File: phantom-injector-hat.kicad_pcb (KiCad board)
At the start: 2 copper layers, 65 x 44.8 mm, 42 parts, among them J1 Conn_02x20_Odd_Even, J2 Conn_02x03_Top_Bottom, J3 Conn_01x03, J4 Conn_01x03, SW1 SW_SPST, U1 LT8362EMSE-PBF

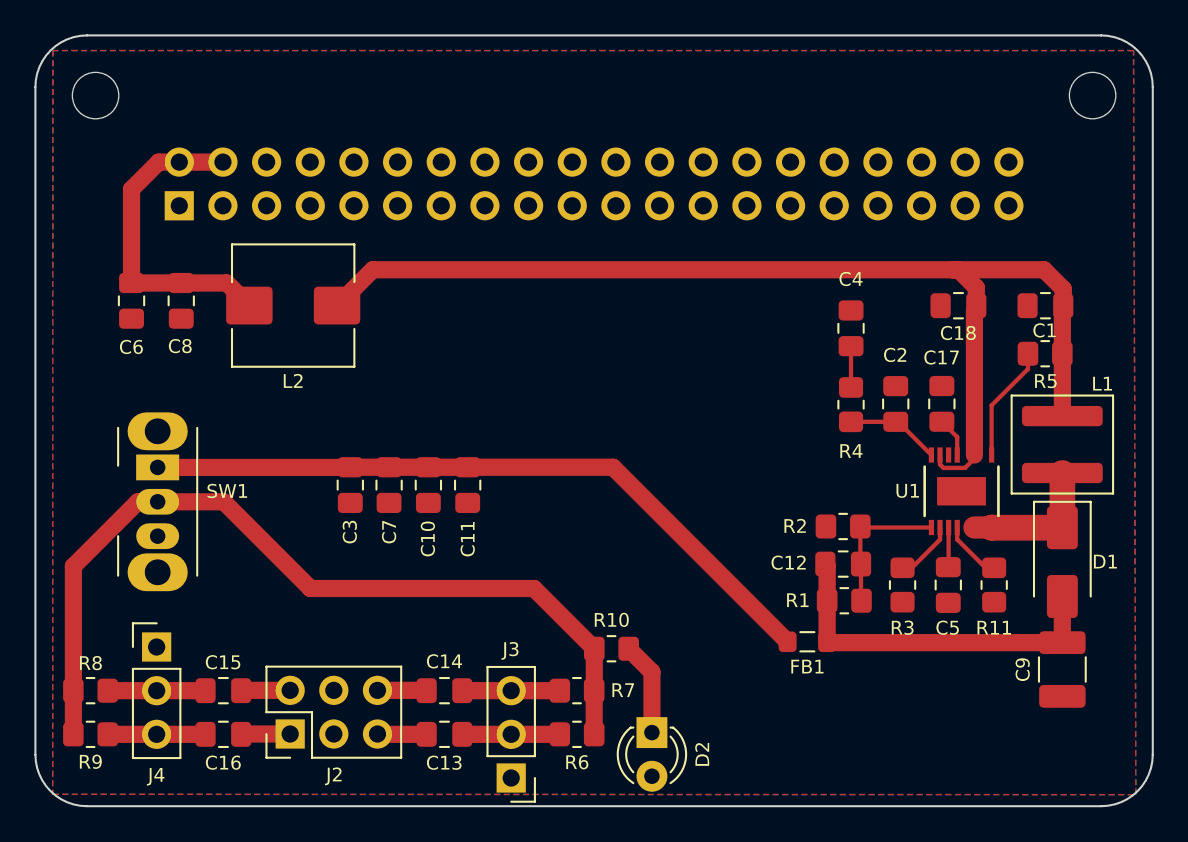
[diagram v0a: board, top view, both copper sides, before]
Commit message: WIP
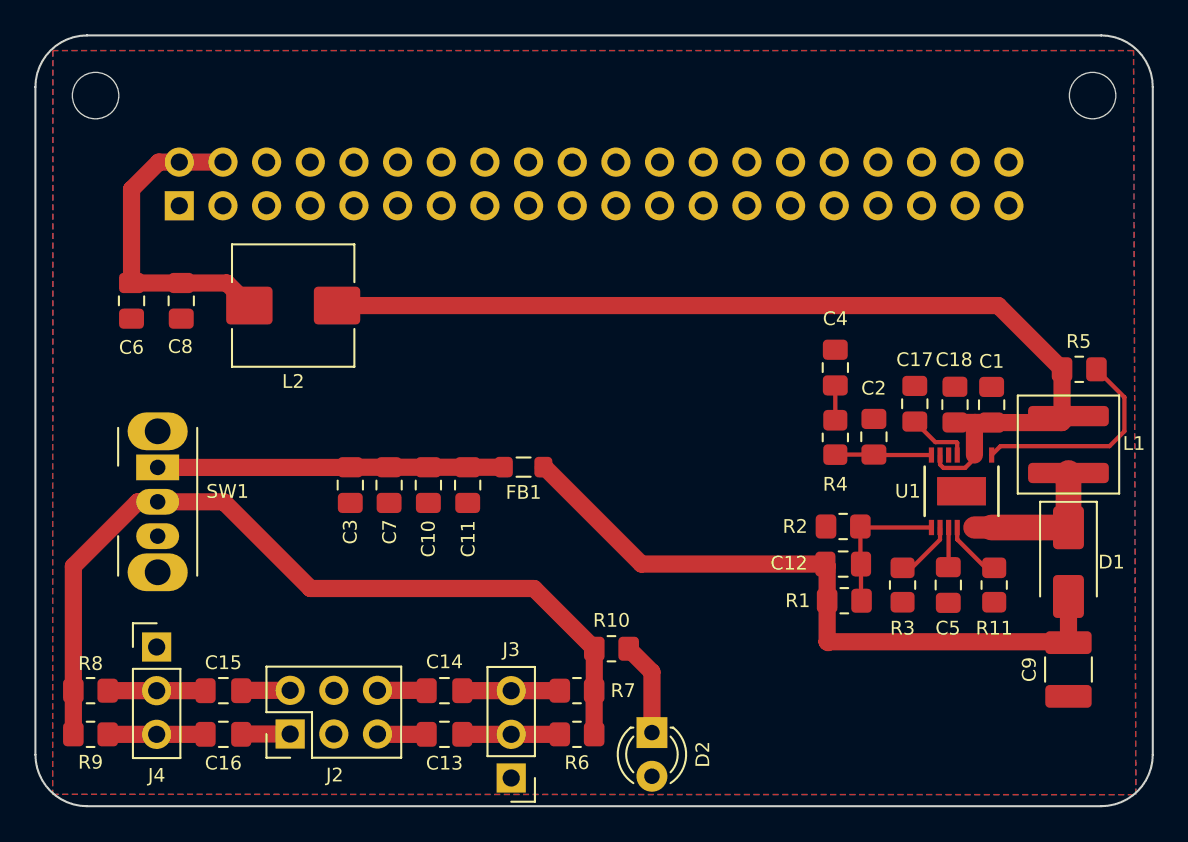
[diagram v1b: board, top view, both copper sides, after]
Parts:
- moved FB1 19.4 mm to (128.4, 69.1)
- moved C1 6.56 mm to (155.6, 65.5), turned to 90 degrees
- moved C18 5.76 mm to (153.5, 65.5), turned to 90 degrees
- moved C4 2.46 mm to (146.5, 63.3)
- moved C2 2.29 mm to (148.8, 67.3)
- moved R5 2.18 mm to (160.7, 63.4), turned to 180 degrees
- moved R4 2.11 mm to (146.5, 67.4)
- moved C17 1.57 mm to (151.2, 65.4)
- moved C9 0.36 mm to (160.1, 80.9)
- moved D1 0.36 mm to (160.1, 74.6)
- moved L1 0.36 mm to (160.1, 67.8)
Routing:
- net /+48V: track 40.9 -> 20.1 mm
- net /+48V_RAW: track 21.0 -> 40.1 mm
- net /+5V_FILT: track 65.7 -> 58.3 mm
- net /EN_UVLO: track 6.77 -> 12.6 mm
- net /INTVCC: track 2.31 -> 3.69 mm
